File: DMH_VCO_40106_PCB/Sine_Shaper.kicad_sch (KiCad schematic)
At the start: 13 parts, among them Q5 BC548, Q6 BC548, U3 TL074

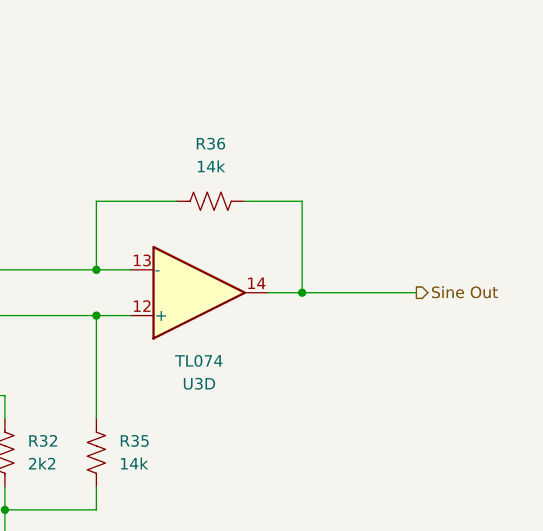
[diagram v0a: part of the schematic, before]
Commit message: Component placement ongoing
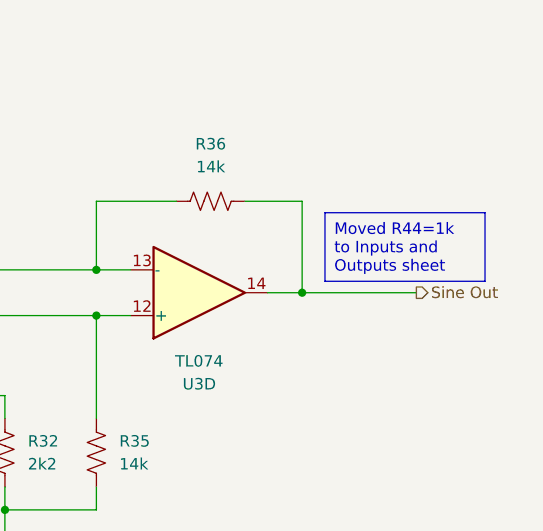
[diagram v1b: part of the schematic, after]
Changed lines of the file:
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@@
+		)
+	)
+	(text_box "Moved R44=1k to Inputs and Outputs sheet"
+		(exclude_from_sim no)
+		(at 179.07 67.31 0)
+		(size 17.78 7.62)
+		(stroke
+			(width 0)
+			(type default)
+		)
+		(fill
+			(type none)
+		)
+		(effects
+			(font
+				(size 1.27 1.27)
+			)
+			(justify left)
 		)
 	)
